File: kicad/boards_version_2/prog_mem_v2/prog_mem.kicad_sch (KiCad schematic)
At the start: 39 parts

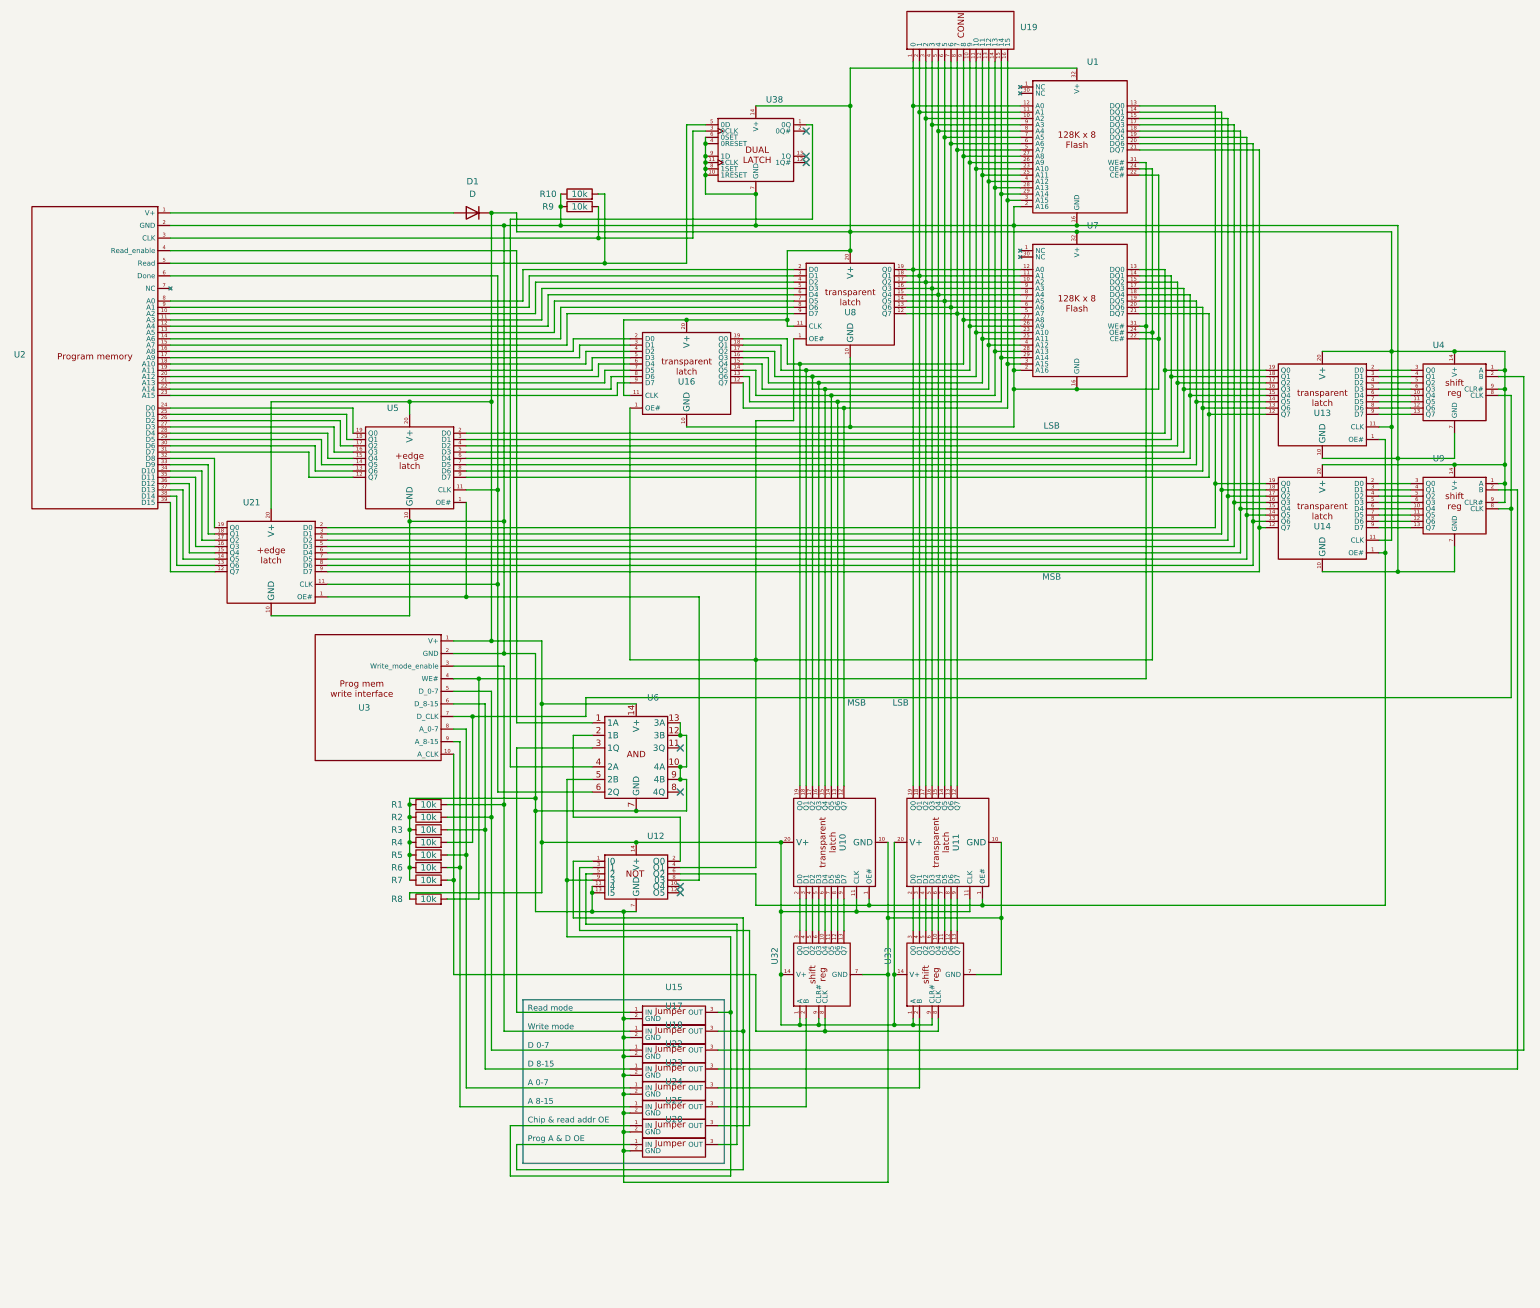
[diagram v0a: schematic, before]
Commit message: Prog mem verified
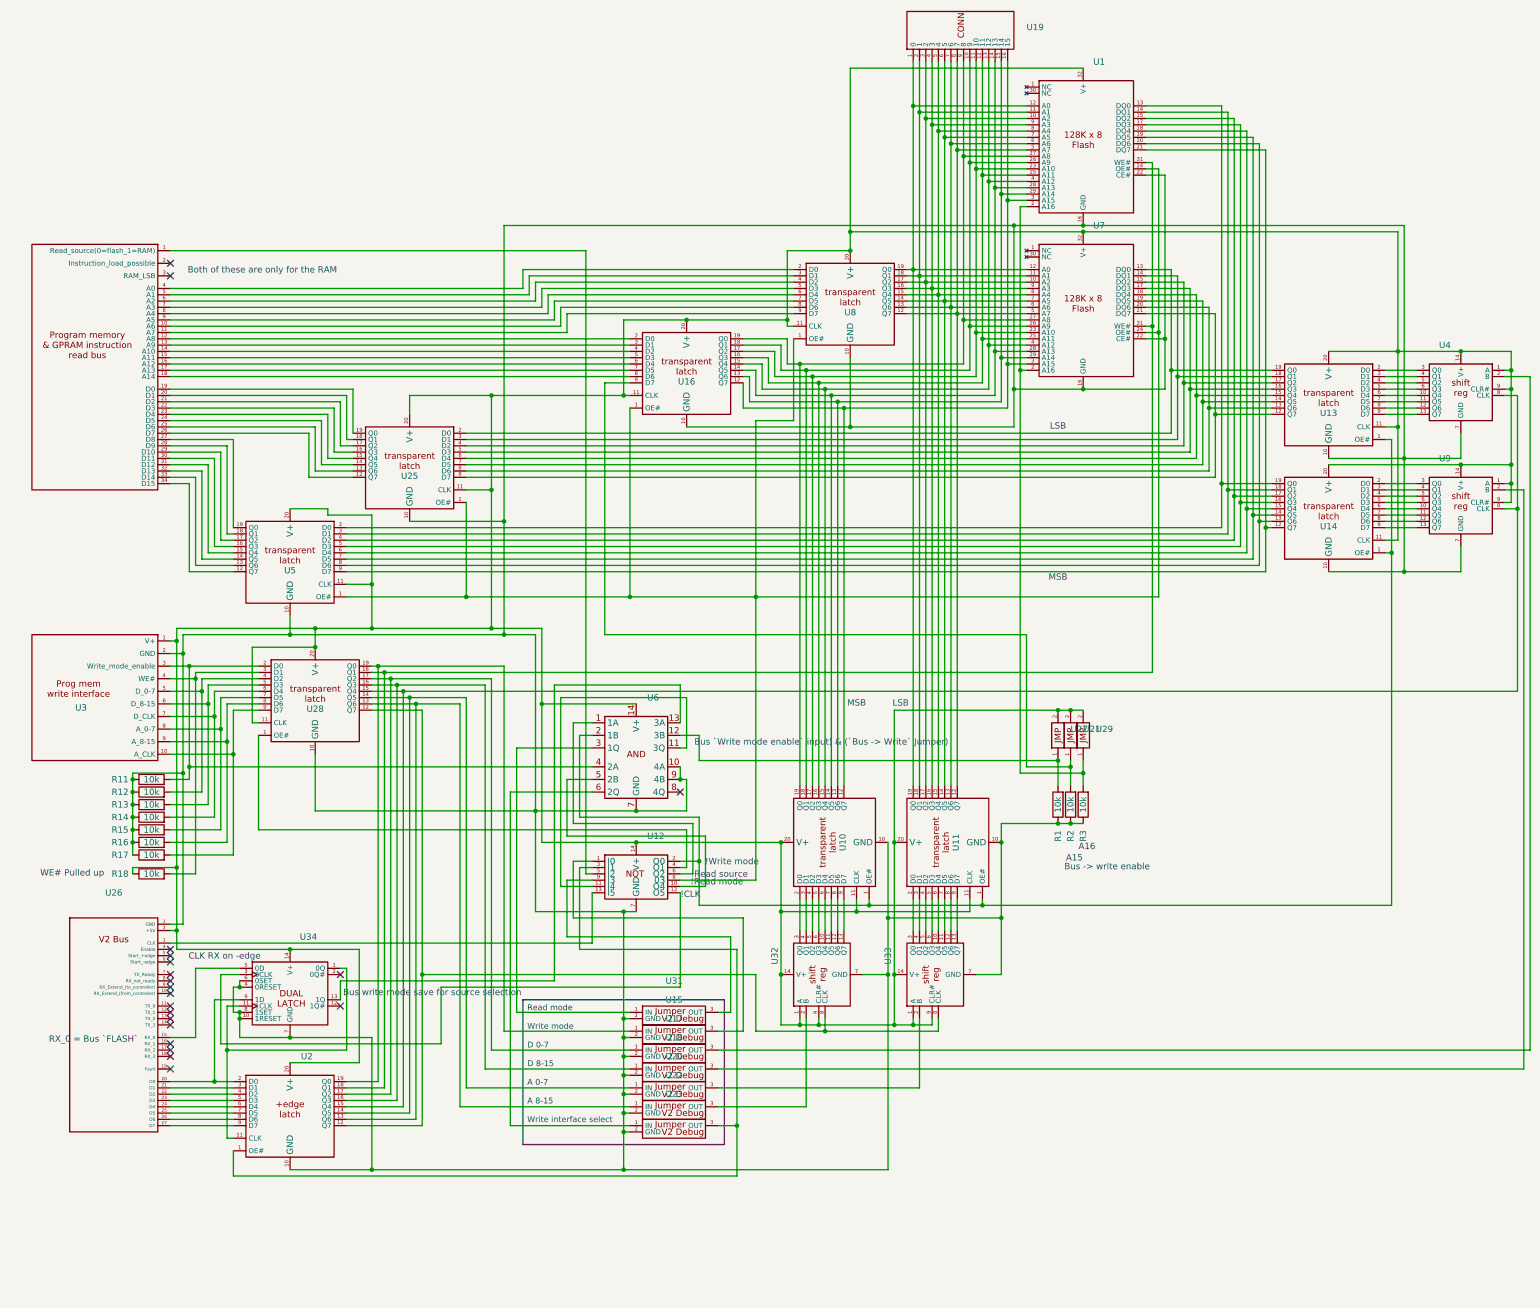
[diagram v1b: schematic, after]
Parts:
- removed D1: D, Diode_THT:D_A-405_P7.62mm_Horizontal, symbol Device:D
- removed R10, R4, R5, R6, R7, R8, R9: 10k, custom_footprint_library:0.4_pitch_resistor, symbol Device:R
- removed U15, U17, U18, U20, U22, U23, U24, U25: ~, custom_footprint_library:jumper, symbol custom_symbol_lib:jumper
- removed U2: ~, Connector_PinHeader_2.54mm:PinHeader_1x39_P2.54mm_Vertical, symbol custom_symbol_lib:prog_mem_interface_read
- removed U21, U5: ~, Package_DIP:DIP-20_W7.62mm, symbol custom_symbol_lib:rising_edge_8_bit_latch
- removed U38: ~, Package_DIP:DIP-14_W7.62mm, symbol custom_symbol_lib:dual_latch
- added R11, R12, R13, R14, R15, R16, R17, R18: 10k, custom_footprint_library:0.4_pitch_resistor, symbol Device:R
- added U15, U17, U18, U20, U22, U23, U31: ~, custom_footprint_library:jumper_v2_gnd_debug_footprint, symbol custom_symbol_lib:jumper_v2_gnd_debug
- added U2: ~, Package_DIP:DIP-20_W7.62mm, symbol custom_symbol_lib:rising_edge_8_bit_latch
- added U21, U27, U29: ~, Connector_PinHeader_2.54mm:PinHeader_1x02_P2.54mm_Vertical, symbol custom_symbol_lib:simple_jumper
- added U25, U28, U5: ~, Package_DIP:DIP-20_W7.62mm, symbol custom_symbol_lib:8_bit_transparent_latch
- added U26: ~, Connector_PinHeader_2.54mm:PinHeader_1x27_P2.54mm_Vertical, symbol custom_symbol_lib:bus_v2
- added U30: ~, Connector_PinHeader_2.54mm:PinHeader_1x34_P2.54mm_Vertical, symbol custom_symbol_lib:prog_mem_read_bus_v2
- added U34: ~, Package_DIP:DIP-14_W7.62mm, symbol custom_symbol_lib:dual_latch
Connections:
- net at R1.1, R2.1, R3.1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: now also R11.1, R12.1, R13.1, R14.1, R15.1, R16.1, R17.1, U15.2 (GND), U17.2 (GND), U18.2 (GND), U2.10 (GND), U20.2 (GND), U22.2 (GND), U23.2 (GND), U25.10 (GND), U26.1 (GND), U28.10 (GND), U31.2 (GND), U34.10 (1RESET), U34.4 (0RESET), U34.6 (0SET), U34.7 (GND), U34.8 (1SET), U5.10 (GND); no longer U1.2 (A16), U12.11 (I4), U12.13 (I5), U6.12 (3B), U6.13 (3A), U7.2 (A16)
- net at U3.5 (D_0-7): now also R12.2, U28.4 (D2); no longer R2.2
- net at U4.2 (B): now also U17.3 (OUT)
- net at U6.5 (2B): now also U12.10 (O4); no longer U12.9 (I3)
- net at U12.3 (I1): now also U2.1 (OE#), U23.3 (OUT)
- net at U6.4 (2A): now also U3.3 (Write_mode_enable), R11.2, U28.2 (D0)
- net at U1.32 (V+), U10.11 (CLK), U10.20 (V+)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: now also R18.1, U2.20 (V+), U21.2, U25.11 (CLK), U25.20 (V+), U26.2 (+5V), U27.2, U28.11 (CLK), U28.20 (V+), U29.2, U34.14 (V+), U5.11 (CLK), U5.20 (V+)
- net at U3.6 (D_8-15): now also R13.2, U28.5 (D3); no longer R3.2
- net at U9.2 (B): now also U18.3 (OUT)
- net at U6.3 (1Q): now also U31.1 (IN)
- net at U1.24 (OE#), U16.1 (OE#), U7.24 (OE#)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: now also U12.8 (03), U25.1 (OE#), U5.1 (OE#); no longer U12.4 (O1)
- net at U8.2 (D0): now also U30.4 (A0)
- net at U8.3 (D1): now also U30.5 (A1)
- net at U8.4 (D2): now also U30.6 (A2)
- net at U8.5 (D3): now also U30.7 (A3)
- net at U8.6 (D4): now also U30.8 (A4)
- net at U8.7 (D5): now also U30.9 (A5)
- net at U8.8 (D6): now also U30.10 (A6)
- net at U8.9 (D7): now also U30.11 (A7)
- net at U6.6 (2Q): now also U23.1 (IN)
- net at U1.13 (DQ0), U14.19 (Q0): now also U5.2 (D0)
- net at U1.14 (DQ1), U14.18 (Q1): now also U5.3 (D1)
- net at U1.15 (DQ2), U14.17 (Q2): now also U5.4 (D2)
- net at U1.17 (DQ3), U14.16 (Q3): now also U5.5 (D3)
- net at U1.18 (DQ4), U14.15 (Q4): now also U5.6 (D4)
- net at U1.19 (DQ5), U14.14 (Q5): now also U5.7 (D5)
- net at U1.20 (DQ6), U14.13 (Q6): now also U5.8 (D6)
- net at U1.21 (DQ7), U14.12 (Q7): now also U5.9 (D7)
- net at U3.9 (A_8-15): now also R16.2, U28.8 (D6)
- net at U32.2 (B): now also U22.3 (OUT)
- net at U3.8 (A_0-7): now also R15.2, U28.7 (D5)
- net at U1.31 (WE#), U7.31 (WE#): now also U2.18 (Q1), U28.18 (Q1); no longer U3.4 (WE#)
- net at U12.1 (I0): now also U15.3 (OUT)
- net at U12.12 (O5): now also U34.3 (0CLK)
- net at U12.2 (O0), U6.2 (1B): now also U10.1 (OE#), U11.1 (OE#), U13.1 (OE#), U14.1 (OE#)
- net at U12.5 (I2): now also U30.1 (Read_source(0=flash_1=RAM))
- net at U4.8 (CLK), U9.8 (CLK): now also U2.15 (Q4), U28.15 (Q4); no longer U3.7 (D_CLK)
- net at U16.2 (D0): now also U30.12 (A8)
- net at U16.3 (D1): now also U30.13 (A9)
- net at U16.4 (D2): now also U30.14 (A10)
- net at U16.5 (D3): now also U30.15 (A11)
- net at U16.6 (D4): now also U30.16 (A12)
- net at U16.7 (D5): now also U30.17 (A13)
- net at U16.8 (D6): now also U30.18 (A14)
- net at U16.9 (D7): now also R2.2, U21.1
- net at U6.1 (1A): now also U12.6 (O2)
- net at U6.11 (3Q): now also U12.11 (I4)
- net at U32.8 (CLK), U33.8 (CLK): now also U2.12 (Q7), U28.12 (Q7); no longer U3.10 (A_CLK)
- net at R1.2: now also U6.12 (3B), U27.1; no longer U3.3 (Write_mode_enable)
- net at U13.12 (Q7), U7.21 (DQ7): now also U25.9 (D7)
- net at U13.13 (Q6), U7.20 (DQ6): now also U25.8 (D6)
- net at U13.14 (Q5), U7.19 (DQ5): now also U25.7 (D5)
- net at U13.15 (Q4), U7.18 (DQ4): now also U25.6 (D4)
- net at U13.16 (Q3), U7.17 (DQ3): now also U25.5 (D3)
- net at U13.17 (Q2), U7.15 (DQ2): now also U25.4 (D2)
- net at U13.18 (Q1), U7.14 (DQ1): now also U25.3 (D1)
- net at U13.19 (Q0), U7.13 (DQ0): now also U25.2 (D0)
- net at U33.2 (B): now also U20.3 (OUT)
- new net: U12.4 (O1), U28.1 (OE#)
- new net: U2.13 (Q6), U22.1 (IN), U28.13 (Q6)
- new net: U2.14 (Q5), U20.1 (IN), U28.14 (Q5)
- new net: U18.1 (IN), U2.16 (Q3), U28.16 (Q3)
- new net: U17.1 (IN), U2.17 (Q2), U28.17 (Q2)
- new net: U15.1 (IN), U2.19 (Q0), U28.19 (Q0)
- new net: R18.2, U28.3 (D1), U3.4 (WE#)
- new net: R14.2, U28.6 (D4), U3.7 (D_CLK)
- new net: R17.2, U28.9 (D7), U3.10 (A_CLK)
- new net: R3.2, U1.2 (A16), U29.1, U7.2 (A16)
- new net: U2.11 (CLK), U34.1 (0Q), U34.11 (1CLK)
- new net: U34.13 (1Q), U6.13 (3A)
- new net: U26.15 (RX_0), U34.5 (0D)
- new net: U2.2 (D0), U26.20 (D0), U34.9 (1D)
- new net: U2.3 (D1), U26.21 (D1)
- new net: U2.4 (D2), U26.22 (D2)
- new net: U2.5 (D3), U26.23 (D3)
- new net: U2.6 (D4), U26.24 (D4)
- new net: U2.7 (D5), U26.25 (D5)
- new net: U2.8 (D6), U26.26 (D6)
- new net: U2.9 (D7), U26.27 (D7)
- new net: U12.13 (I5), U26.3 (CLK)
- new net: U25.19 (Q0), U30.19 (D0)
- new net: U25.18 (Q1), U30.20 (D1)
- new net: U25.17 (Q2), U30.21 (D2)
- new net: U25.16 (Q3), U30.22 (D3)
- new net: U25.15 (Q4), U30.23 (D4)
- new net: U25.14 (Q5), U30.24 (D5)
- new net: U25.13 (Q6), U30.25 (D6)
- new net: U25.12 (Q7), U30.26 (D7)
- new net: U30.27 (D8), U5.19 (Q0)
- new net: U30.28 (D9), U5.18 (Q1)
- new net: U30.29 (D10), U5.17 (Q2)
- new net: U30.30 (D11), U5.16 (Q3)
- new net: U30.31 (D12), U5.15 (Q4)
- new net: U30.32 (D13), U5.14 (Q5)
- new net: U30.33 (D14), U5.13 (Q6)
- new net: U30.34 (D15), U5.12 (Q7)
- new net: U12.9 (I3), U31.3 (OUT)
- no-connect marks 7 -> 20
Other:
- note added: "!CLK"
- note added: "!Read mode"
- note added: "!Read source"
- note added: "!Write mode"
- note added: "A15"
- note added: "A16"
- note added: "Both of these are only for the RAM"
- note added: "Bus -> write enable"
- note added: "Bus `Write mode enable` input) & (`Bus -> Write` Jumper)"
- note added: "Bus write mode save for source selection"
- note added: "CLK RX on -edge"
- note added: "RX_0 = Bus `FLASH`"
- note added: "WE# Pulled up"
- moved on the sheet: U1, U13, U14, U3, U4, U7, U9

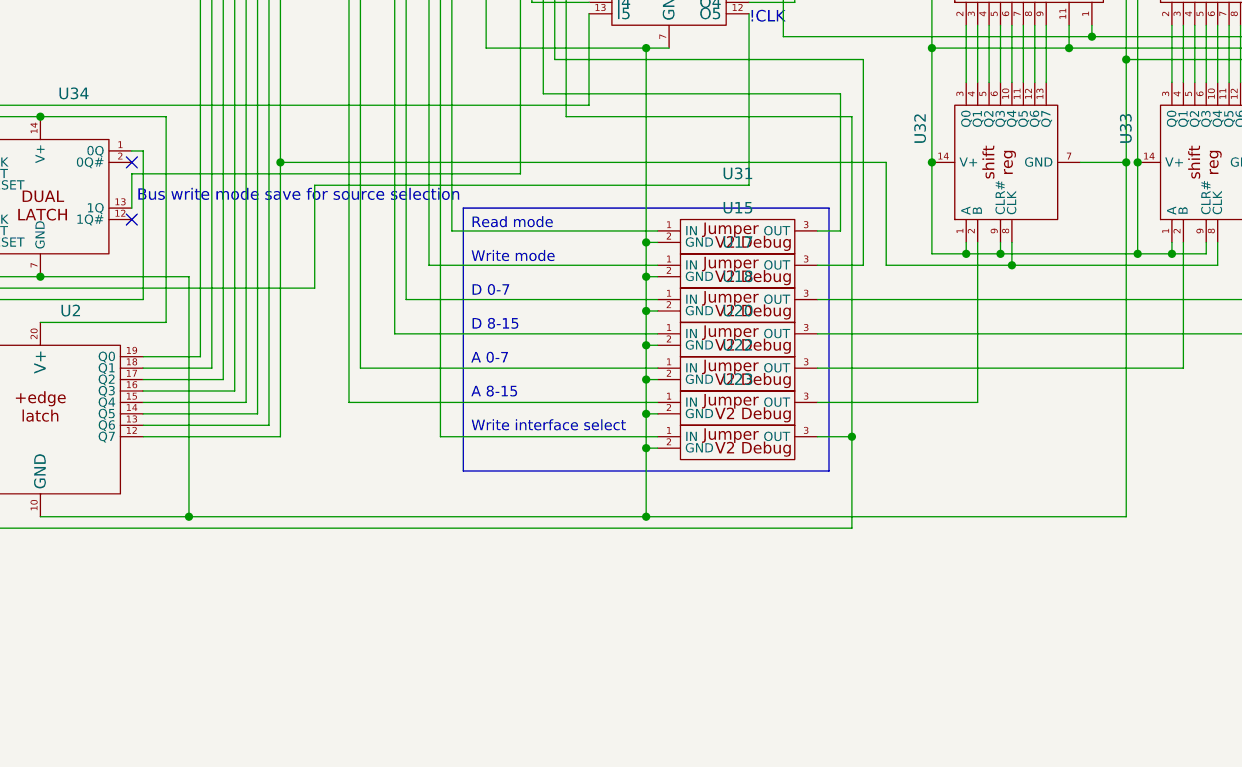
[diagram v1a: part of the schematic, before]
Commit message: Work mostly on bus
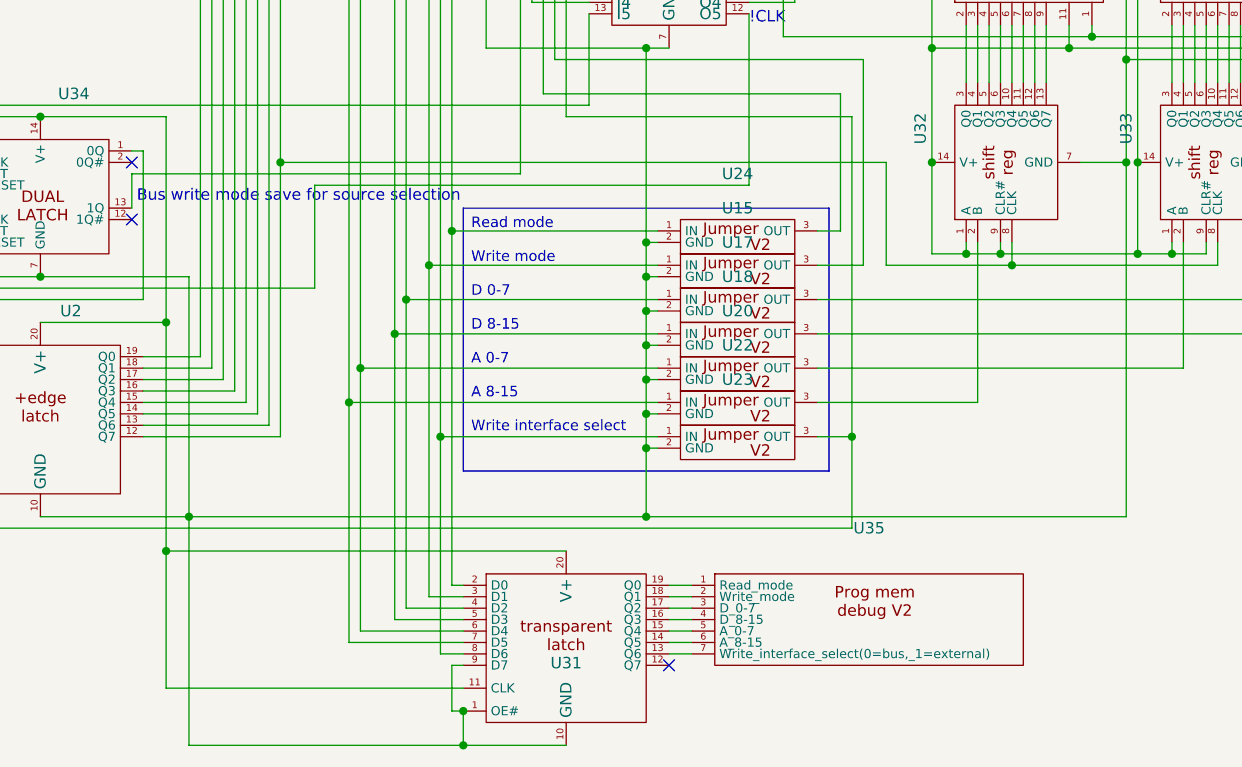
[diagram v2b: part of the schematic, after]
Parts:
- removed U15, U17, U18, U20, U22, U23, U31: ~, custom_footprint_library:jumper_v2_gnd_debug_footprint, symbol custom_symbol_lib:jumper_v2_gnd_debug
- added U15, U17, U18, U20, U22, U23, U24: ~, custom_footprint_library:jumper_v2_gnd_footprint, symbol custom_symbol_lib:jumer_v2_gnd
- added U31: ~, Package_DIP:DIP-20_W7.62mm, symbol custom_symbol_lib:8_bit_transparent_latch
- added U35: ~, Connector_PinHeader_2.54mm:PinHeader_2x04_P2.54mm_Vertical, symbol custom_symbol_lib:debug_v2_prog_mem
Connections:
- net at R1.1, R11.1, R12.1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: now also U15.2 (GND), U17.2 (GND), U18.2 (GND), U20.2 (GND), U22.2 (GND), U23.2 (GND), U24.2 (GND), U31.1 (OE#), U31.10 (GND), U31.9 (D7)
- net at R18.1, U1.32 (V+), U10.11 (CLK)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: now also U31.11 (CLK), U31.20 (V+)
- net at U2.13 (Q6), U28.13 (Q6): now also U22.1 (IN), U31.7 (D5)
- net at U2.14 (Q5), U28.14 (Q5): now also U20.1 (IN), U31.6 (D4)
- net at U2.16 (Q3), U28.16 (Q3): now also U18.1 (IN), U31.5 (D3)
- net at U2.17 (Q2), U28.17 (Q2): now also U17.1 (IN), U31.4 (D2)
- net at U2.19 (Q0), U28.19 (Q0): now also U15.1 (IN), U31.3 (D1)
- net at U6.6 (2Q): now also U23.1 (IN), U31.8 (D6)
- net at U12.3 (I1), U2.1 (OE#): now also U23.3 (OUT)
- net at U12.1 (I0): now also U15.3 (OUT)
- net at U12.9 (I3): now also U24.3 (OUT)
- net at U9.2 (B): now also U18.3 (OUT)
- net at U6.3 (1Q): now also U24.1 (IN), U31.2 (D0)
- net at U4.2 (B): now also U17.3 (OUT)
- net at U32.2 (B): now also U22.3 (OUT)
- net at U33.2 (B): now also U20.3 (OUT)
- new net: U31.13 (Q6), U35.7 (Write_interface_select(0=bus,_1=external))
- new net: U31.14 (Q5), U35.6 (A_8-15)
- new net: U31.15 (Q4), U35.5 (A_0-7)
- new net: U31.16 (Q3), U35.4 (D_8-15)
- new net: U31.17 (Q2), U35.3 (D_0-7)
- new net: U31.18 (Q1), U35.2 (Write_mode)
- new net: U31.19 (Q0), U35.1 (Read_mode)
- no-connect marks 20 -> 21
